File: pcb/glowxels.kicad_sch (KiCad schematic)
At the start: 79 parts, among them J1 OUT, J2 IN, U1 STP16CPC26, U2 STP16CPC26, U3 STP16CPC26, U4 STP16CPC26

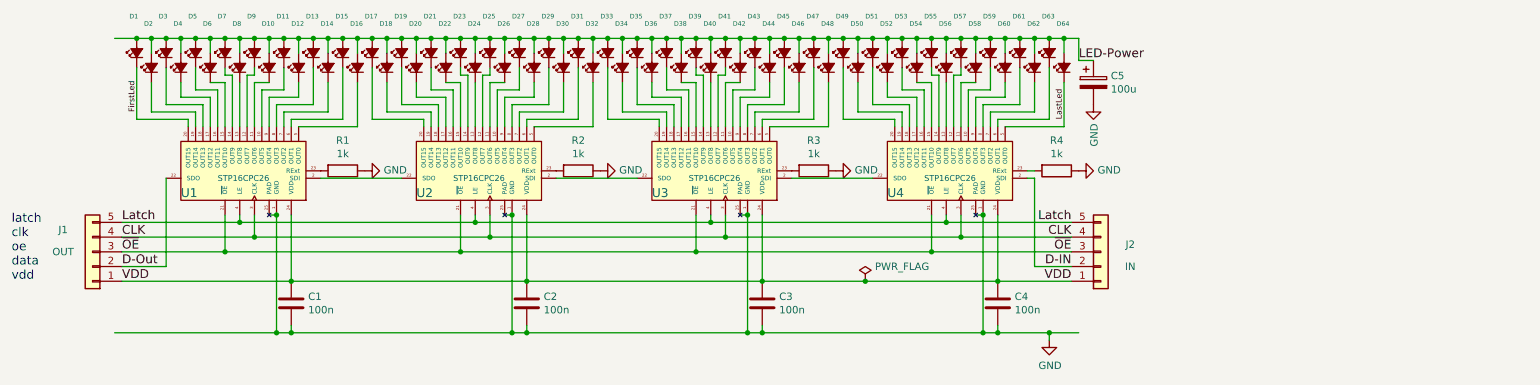
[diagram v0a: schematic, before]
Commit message: First version, fully routed.
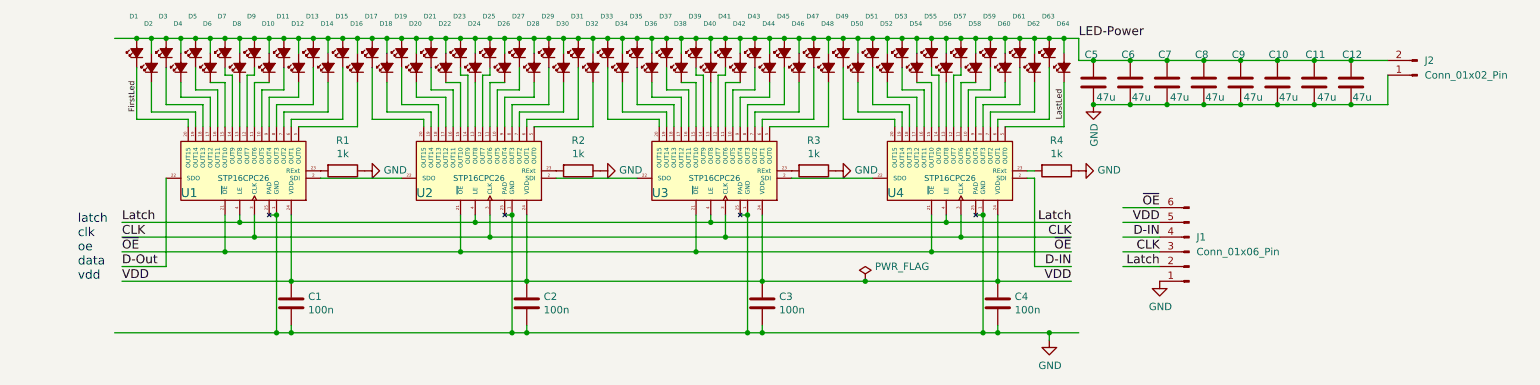
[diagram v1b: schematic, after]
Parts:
- removed C5: 100u, Capacitor_SMD:CP_Elec_6.3x5.3, symbol Device:CP
- removed J1: OUT, Glowxels:EdgeConnect, symbol Connector_Generic:Conn_01x05
- removed J2: IN, Glowxels:EdgeConnect, symbol Connector_Generic:Conn_01x05
- added C10, C11, C12, C5, C6, C7, C8, C9: 47u, Capacitor_SMD:C_1210_3225Metric, symbol Device:C
- added J1: Conn_01x06_Pin, Connector_PinHeader_2.00mm:PinHeader_1x06_P2.00mm_Vertical, symbol Connector:Conn_01x06_Pin
- added J2: Conn_01x02_Pin, Connector_PinHeader_2.00mm:PinHeader_1x02_P2.00mm_Vertical, symbol Connector:Conn_01x02_Pin
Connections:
- net CLK: now also J1.3 (Pin_3)
- net D-IN: now also J1.4 (Pin_4)
- net GND: now also C10.2, C11.2, C12.2, C5.2, C6.2, C7.2, C8.2, C9.2, J1.1 (Pin_1), J2.1 (Pin_1)
- net LED-Power: now also C10.1, C11.1, C12.1, C5.1, C6.1, C7.1, C8.1, C9.1, J2.2 (Pin_2)
- net Latch: now also J1.2 (Pin_2)
- net VDD: now also J1.5 (Pin_5)
- net ~{OE}: now also J1.6 (Pin_6)
